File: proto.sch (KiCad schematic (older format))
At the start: 146 parts, among them SW1 SW_Push, U1 ATmega32U4-AU, Y1 16MHz

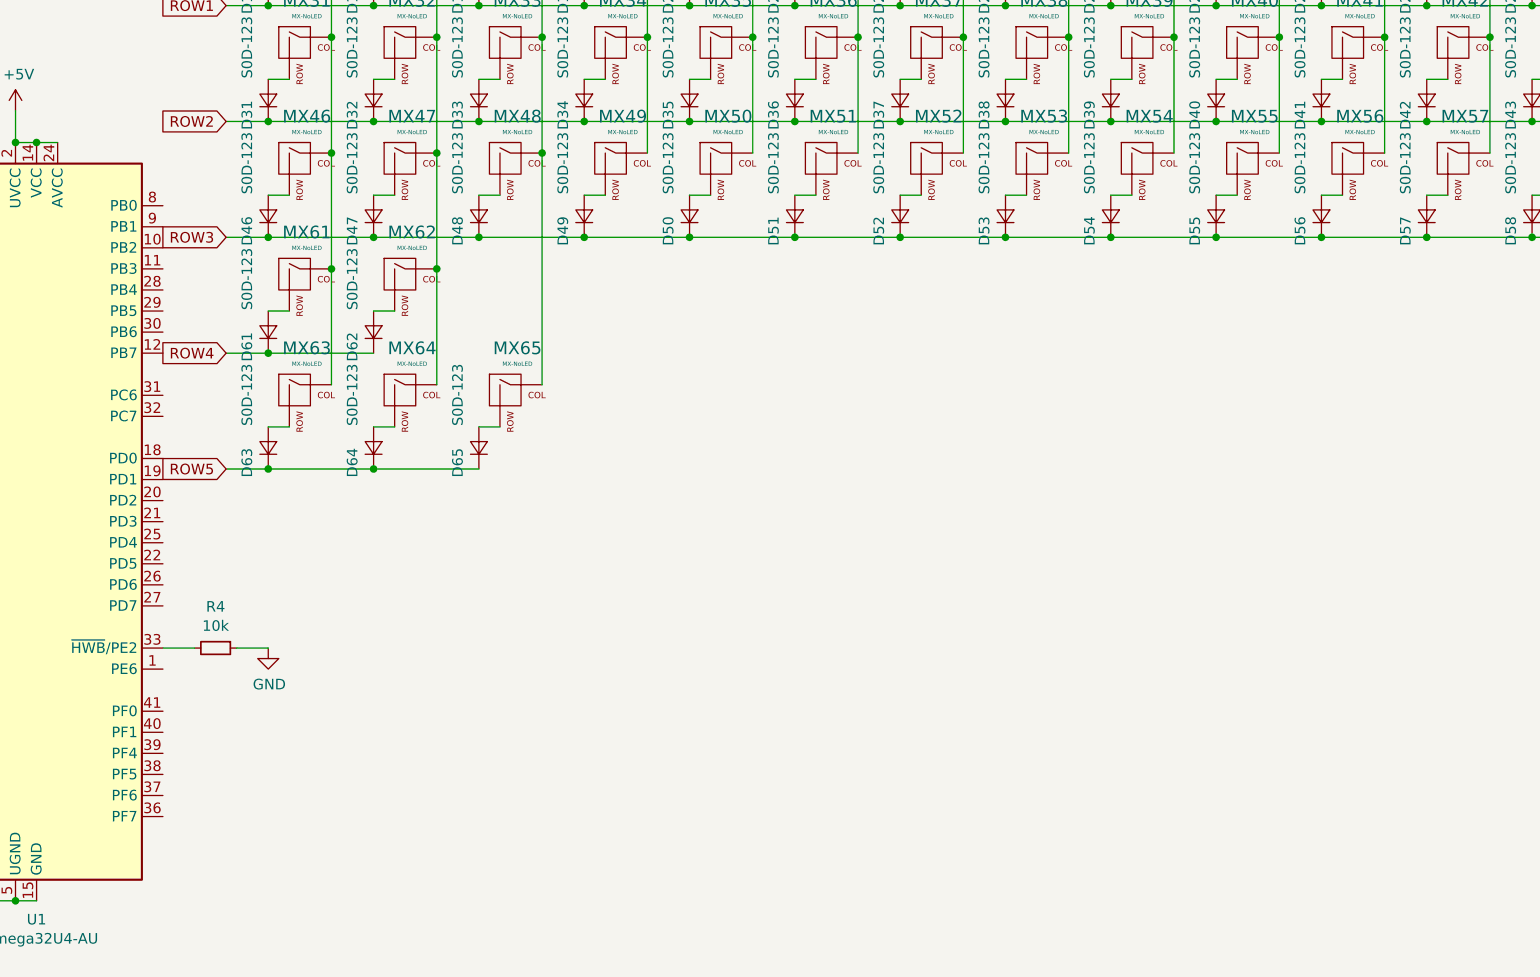
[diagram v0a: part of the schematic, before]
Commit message: routing
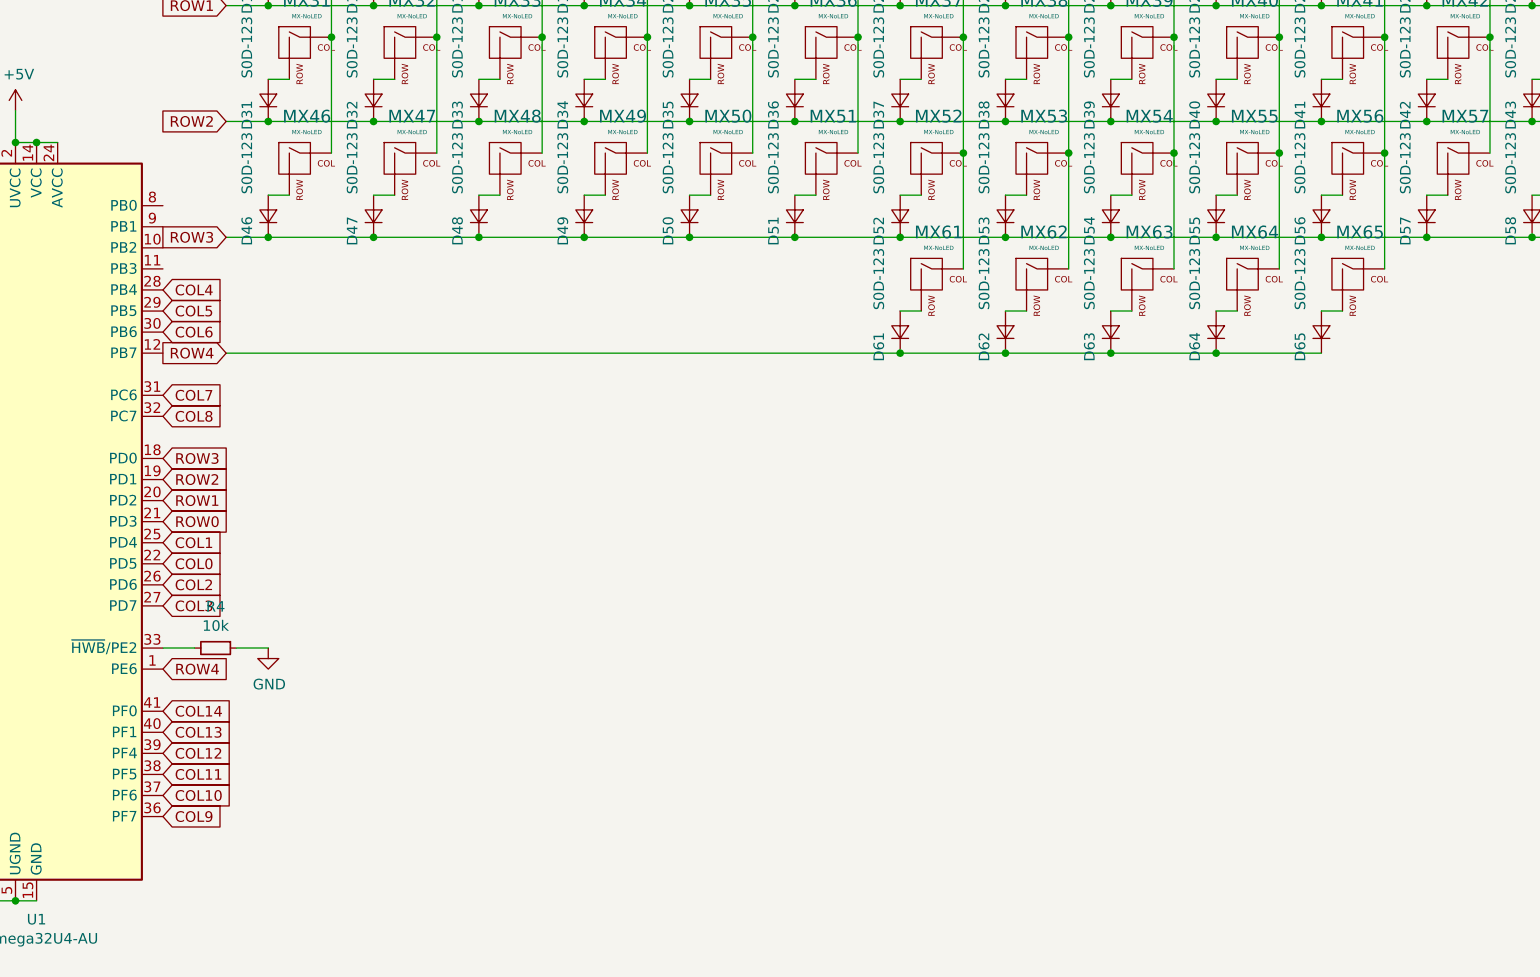
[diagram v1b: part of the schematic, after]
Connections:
- net ROW5 is gone; now on net ROW4: D63.1 (K), D64.1 (K), D65.1 (K)
- net COL0: now also U1.22 (PD5); no longer MX61.1 (COL), MX63.1 (COL)
- net COL1: now also U1.25 (PD4); no longer MX62.1 (COL), MX64.1 (COL)
- net COL10: now also MX65.1 (COL), U1.37 (PF6)
- net COL11: now also U1.38 (PF5)
- net COL12: now also U1.39 (PF4)
- net COL13: now also U1.40 (PF1)
- net COL14: now also U1.41 (PF0)
- net COL2: now also U1.26 (PD6); no longer MX65.1 (COL)
- net COL3: now also U1.27 (PD7)
- net COL4: now also U1.28 (PB4)
- net COL5: now also U1.29 (PB5)
- net COL6: now also MX61.1 (COL), U1.30 (PB6)
- net COL7: now also MX62.1 (COL), U1.31 (PC6)
- net COL8: now also MX63.1 (COL), U1.32 (PC7)
- net COL9: now also MX64.1 (COL), U1.36 (PF7)
- net ROW0: now also U1.21 (PD3)
- net ROW1: now also U1.20 (PD2)
- net ROW2: now also U1.19 (PD1)
- net ROW3: now also U1.18 (PD0)
- net ROW4: now also U1.1 (PE6)
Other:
- moved on the sheet: D61, D62, D63, D64, D65, MX61, MX62, MX63, MX64, MX65
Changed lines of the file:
@@
 EESchema Schematic File Version 4
+LIBS:proto-cache
 EELAYER 30 0
 EELAYER END
@@
 $EndComp
 Wire Wire Line
-	3850 3700 3950 3700
+	6850 3700 6950 3700
 $Comp
 L Device:D_Small D61
 U 1 1 601863FD
-P 3850 3800
-F 0 "D61" H 3850 3900 50  0000 R CNN
-F 1 "S0D-123" H 4250 3900 50  0000 R CNN
-F 2 "Diode_SMD:D_SOD-123" V 3850 3800 50  0001 C CNN
-F 3 "~" V 3850 3800 50  0001 C CNN
-	1    3850 3800
+P 6850 3800
+F 0 "D61" H 6850 3900 50  0000 R CNN
+F 1 "S0D-123" H 7250 3900 50  0000 R CNN
+F 2 "Diode_SMD:D_SOD-123" V 6850 3800 50  0001 C CNN
+F 3 "~" V 6850 3800 50  0001 C CNN
+	1    6850 3800
 	0    -1   -1   0
 $EndComp
@@
 L MX_Alps_Hybrid:MX-NoLED MX61
 U 1 1 60186407
-P 4000 3550
-F 0 "MX61" H 4033 3773 60  0000 C CNN
-F 1 "MX-NoLED" H 4033 3699 20  0000 C CNN
-F 2 "MX_Alps_Hybrid:MX-1U" H 3375 3525 60  0001 C CNN
-F 3 "" H 3375 3525 60  0001 C CNN
-	1    4000 3550
-	1    0    0    -1
-$EndComp
-Wire Wire Line
-	3850 4250 3950 4250
+P 7000 3550
+F 0 "MX61" H 7033 3773 60  0000 C CNN
+F 1 "MX-NoLED" H 7033 3699 20  0000 C CNN
+F 2 "MX_Alps_Hybrid:MX-1U" H 6375 3525 60  0001 C CNN
+F 3 "" H 6375 3525 60  0001 C CNN
+	1    7000 3550
+	1    0    0    -1
+$EndComp
+Wire Wire Line
+	7850 3700 7950 3700
 $Comp
 L Device:D_Small D63
 U 1 1 60186412
-P 3850 4350
-F 0 "D63" H 3850 4450 50  0000 R CNN
-F 1 "S0D-123" H 4250 4450 50  0000 R CNN
-F 2 "Diode_SMD:D_SOD-123" V 3850 4350 50  0001 C CNN
-F 3 "~" V 3850 4350 50  0001 C CNN
-	1    3850 4350
+P 7850 3800
+F 0 "D63" H 7850 3900 50  0000 R CNN
+F 1 "S0D-123" H 8250 3900 50  0000 R CNN
+F 2 "Diode_SMD:D_SOD-123" V 7850 3800 50  0001 C CNN
+F 3 "~" V 7850 3800 50  0001 C CNN
+	1    7850 3800
 	0    -1   -1   0
 $EndComp
@@
 L MX_Alps_Hybrid:MX-NoLED MX63
 U 1 1 6018641C
-P 4000 4100
-F 0 "MX63" H 4033 4323 60  0000 C CNN
-F 1 "MX-NoLED" H 4033 4249 20  0000 C CNN
-F 2 "MX_Alps_Hybrid:MX-1U" H 3375 4075 60  0001 C CNN
-F 3 "" H 3375 4075 60  0001 C CNN
-	1    4000 4100
+P 8000 3550
+F 0 "MX63" H 8033 3773 60  0000 C CNN
+F 1 "MX-NoLED" H 8033 3699 20  0000 C CNN
+F 2 "MX_Alps_Hybrid:MX-1U" H 7375 3525 60  0001 C CNN
+F 3 "" H 7375 3525 60  0001 C CNN
+	1    8000 3550
 	1    0    0    -1
 $EndComp
@@
 $EndComp
 Wire Wire Line
-	4350 3700 4450 3700
+	7350 3700 7450 3700
 $Comp
 L Device:D_Small D62
 U 1 1 6022FD4C
-P 4350 3800
-F 0 "D62" H 4350 3900 50  0000 R CNN
-F 1 "S0D-123" H 4750 3900 50  0000 R CNN
-F 2 "Diode_SMD:D_SOD-123" V 4350 3800 50  0001 C CNN
-F 3 "~" V 4350 3800 50  0001 C CNN
-	1    4350 3800
+P 7350 3800
+F 0 "D62" H 7350 3900 50  0000 R CNN
+F 1 "S0D-123" H 7750 3900 50  0000 R CNN
+F 2 "Diode_SMD:D_SOD-123" V 7350 3800 50  0001 C CNN
+F 3 "~" V 7350 3800 50  0001 C CNN
+	1    7350 3800
 	0    -1   -1   0
 $EndComp
@@
 L MX_Alps_Hybrid:MX-NoLED MX62
 U 1 1 6022FD56
-P 4500 3550
-F 0 "MX62" H 4533 3773 60  0000 C CNN
-F 1 "MX-NoLED" H 4533 3699 20  0000 C CNN
-F 2 "MX_Alps_Hybrid:MX-1U" H 3875 3525 60  0001 C CNN
-F 3 "" H 3875 3525 60  0001 C CNN
-	1    4500 3550
-	1    0    0    -1
-$EndComp
-Wire Wire Line
-	4350 4250 4450 4250
+P 7500 3550
+F 0 "MX62" H 7533 3773 60  0000 C CNN
+F 1 "MX-NoLED" H 7533 3699 20  0000 C CNN
+F 2 "MX_Alps_Hybrid:MX-1U" H 6875 3525 60  0001 C CNN
+F 3 "" H 6875 3525 60  0001 C CNN
+	1    7500 3550
+	1    0    0    -1
+$EndComp
+Wire Wire Line
+	8350 3700 8450 3700
 $Comp
 L Device:D_Small D64
 U 1 1 60235738
-P 4350 4350
-F 0 "D64" H 4350 4450 50  0000 R CNN
-F 1 "S0D-123" H 4750 4450 50  0000 R CNN
-F 2 "Diode_SMD:D_SOD-123" V 4350 4350 50  0001 C CNN
-F 3 "~" V 4350 4350 50  0001 C CNN
-	1    4350 4350
+P 8350 3800
+F 0 "D64" H 8350 3900 50  0000 R CNN
+F 1 "S0D-123" H 8750 3900 50  0000 R CNN
+F 2 "Diode_SMD:D_SOD-123" V 8350 3800 50  0001 C CNN
+F 3 "~" V 8350 3800 50  0001 C CNN
+	1    8350 3800
 	0    -1   -1   0
 $EndComp
@@
 L MX_Alps_Hybrid:MX-NoLED MX64
 U 1 1 60235742
-P 4500 4100
-F 0 "MX64" H 4533 4323 60  0000 C CNN
-F 1 "MX-NoLED" H 4533 4249 20  0000 C CNN
-F 2 "MX_Alps_Hybrid:MX-1U" H 3875 4075 60  0001 C CNN
-F 3 "" H 3875 4075 60  0001 C CNN
-	1    4500 4100
-	1    0    0    -1
-$EndComp
-Wire Wire Line
-	4850 4250 4950 4250
+P 8500 3550
+F 0 "MX64" H 8533 3773 60  0000 C CNN
+F 1 "MX-NoLED" H 8533 3699 20  0000 C CNN
+F 2 "MX_Alps_Hybrid:MX-1U" H 7875 3525 60  0001 C CNN
+F 3 "" H 7875 3525 60  0001 C CNN
+	1    8500 3550
+	1    0    0    -1
+$EndComp
+Wire Wire Line
+	8850 3700 8950 3700
 $Comp
 L Device:D_Small D65
 U 1 1 6023574D
-P 4850 4350
-F 0 "D65" H 4850 4450 50  0000 R CNN
-F 1 "S0D-123" H 5250 4450 50  0000 R CNN
-F 2 "Diode_SMD:D_SOD-123" V 4850 4350 50  0001 C CNN
-F 3 "~" V 4850 4350 50  0001 C CNN
-	1    4850 4350
+P 8850 3800
+F 0 "D65" H 8850 3900 50  0000 R CNN
+F 1 "S0D-123" H 9250 3900 50  0000 R CNN
+F 2 "Diode_SMD:D_SOD-123" V 8850 3800 50  0001 C CNN
+F 3 "~" V 8850 3800 50  0001 C CNN
+	1    8850 3800
 	0    -1   -1   0
 $EndComp
@@
 L MX_Alps_Hybrid:MX-NoLED MX65
 U 1 1 60235757
-P 5000 4100
-F 0 "MX65" H 5033 4323 60  0000 C CNN
-F 1 "MX-NoLED" H 5033 4249 20  0000 C CNN
-F 2 "MX_Alps_Hybrid:MX-1U" H 4375 4075 60  0001 C CNN
-F 3 "" H 4375 4075 60  0001 C CNN
-	1    5000 4100
-	1    0    0    -1
-$EndComp
-Wire Wire Line
-	4150 4050 4150 3500
+P 9000 3550
+F 0 "MX65" H 9033 3773 60  0000 C CNN
+F 1 "MX-NoLED" H 9033 3699 20  0000 C CNN
+F 2 "MX_Alps_Hybrid:MX-1U" H 8375 3525 60  0001 C CNN
+F 3 "" H 8375 3525 60  0001 C CNN
+	1    9000 3550
+	1    0    0    -1
+$EndComp
 Connection ~ 4150 1300
 Wire Wire Line
@@
 Wire Wire Line
 	4150 2400 4150 1850
-Connection ~ 4150 2950
 Wire Wire Line
 	4150 2950 4150 2400
-Connection ~ 4150 3500
-Wire Wire Line
-	4150 3500 4150 2950
-Wire Wire Line
-	4650 4050 4650 3500
+Wire Wire Line
+	7150 3500 7150 2950
 Connection ~ 4650 1300
 Wire Wire Line
@@
 Wire Wire Line
 	4650 2400 4650 1850
-Connection ~ 4650 2950
 Wire Wire Line
 	4650 2950 4650 2400
-Connection ~ 4650 3500
-Wire Wire Line
-	4650 3500 4650 2950
-Wire Wire Line
-	5150 4050 5150 2950
+Wire Wire Line
+	7650 3500 7650 2950
 Connection ~ 5150 1300
 Wire Wire Line
@@
 Wire Wire Line
 	5150 2400 5150 1850
-Connection ~ 5150 2950
 Wire Wire Line
 	5150 2950 5150 2400
@@
 	10350 3350 9850 3350
 Wire Wire Line
-	4350 3900 3850 3900
-Connection ~ 3850 3900
-Wire Wire Line
-	3850 3900 3650 3900
-Wire Wire Line
-	4850 4450 4350 4450
-Connection ~ 3850 4450
-Wire Wire Line
-	3850 4450 3650 4450
-Connection ~ 4350 4450
-Wire Wire Line
-	4350 4450 3850 4450
+	8850 3900 8350 3900
+Connection ~ 8350 3900
+Wire Wire Line
+	8350 3900 7850 3900
 Text GLabel 3650 1700 0    50   Input ~ 0
 ROW0
@@
 Text GLabel 3650 3900 0    50   Input ~ 0
 ROW4
-Text GLabel 3650 4450 0    50   Input ~ 0
-ROW5
 Text GLabel 4150 950  1    50   Input ~ 0
 COL0
@@
 Text GLabel 11150 950  1    50   Input ~ 0
 COL14
+Wire Wire Line
+	7350 3900 7850 3900
+Connection ~ 7850 3900
+Wire Wire Line
+	9150 2950 9150 3500
+Wire Wire Line
+	8650 2950 8650 3500
+Wire Wire Line
+	8150 2950 8150 3500
+Text GLabel 3350 4700 2    50   Input ~ 0
+ROW0
+Text GLabel 3350 4600 2    50   Input ~ 0
+ROW1
+Text GLabel 3350 4500 2    50   Input ~ 0
+ROW2
+Text GLabel 3350 4400 2    50   Input ~ 0
+ROW3
+Text GLabel 3350 5400 2    50   Input ~ 0
+ROW4
+Connection ~ 7150 2950
+Connection ~ 7650 2950
+Connection ~ 8150 2950
+Connection ~ 8650 2950
+Connection ~ 9150 2950
+Wire Wire Line
+	7350 3900 6850 3900
+Connection ~ 7350 3900
+Connection ~ 6850 3900
+Wire Wire Line
+	6850 3900 3650 3900
+Text GLabel 3350 4900 2    50   Input ~ 0
+COL0
+Text GLabel 3350 4800 2    50   Input ~ 0
+COL1
+Text GLabel 3350 5000 2    50   Input ~ 0
+COL2
+Text GLabel 3350 5100 2    50   Input ~ 0
+COL3
+Text GLabel 3350 3600 2    50   Input ~ 0
+COL4
+Text GLabel 3350 3700 2    50   Input ~ 0
+COL5
+Text GLabel 3350 3800 2    50   Input ~ 0
+COL6
+Text GLabel 3350 4100 2    50   Input ~ 0
+COL7
+Text GLabel 3350 4200 2    50   Input ~ 0
+COL8
+Text GLabel 3350 6100 2    50   Input ~ 0
+COL9
+Text GLabel 3350 6000 2    50   Input ~ 0
+COL10
+Text GLabel 3350 5900 2    50   Input ~ 0
+COL11
+Text GLabel 3350 5800 2    50   Input ~ 0
+COL12
+Text GLabel 3350 5700 2    50   Input ~ 0
+COL13
+Text GLabel 3350 5600 2    50   Input ~ 0
+COL14
 $EndSCHEMATC
